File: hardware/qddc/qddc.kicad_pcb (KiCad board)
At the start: 2 copper layers, 71.1 x 46.4 mm, 38 parts, among them IC1 FST3253MTCX, IC2 OPA2350UA, J4 PWR, J7 Conn_01x03_Male, T1 ETC4-1-2TR

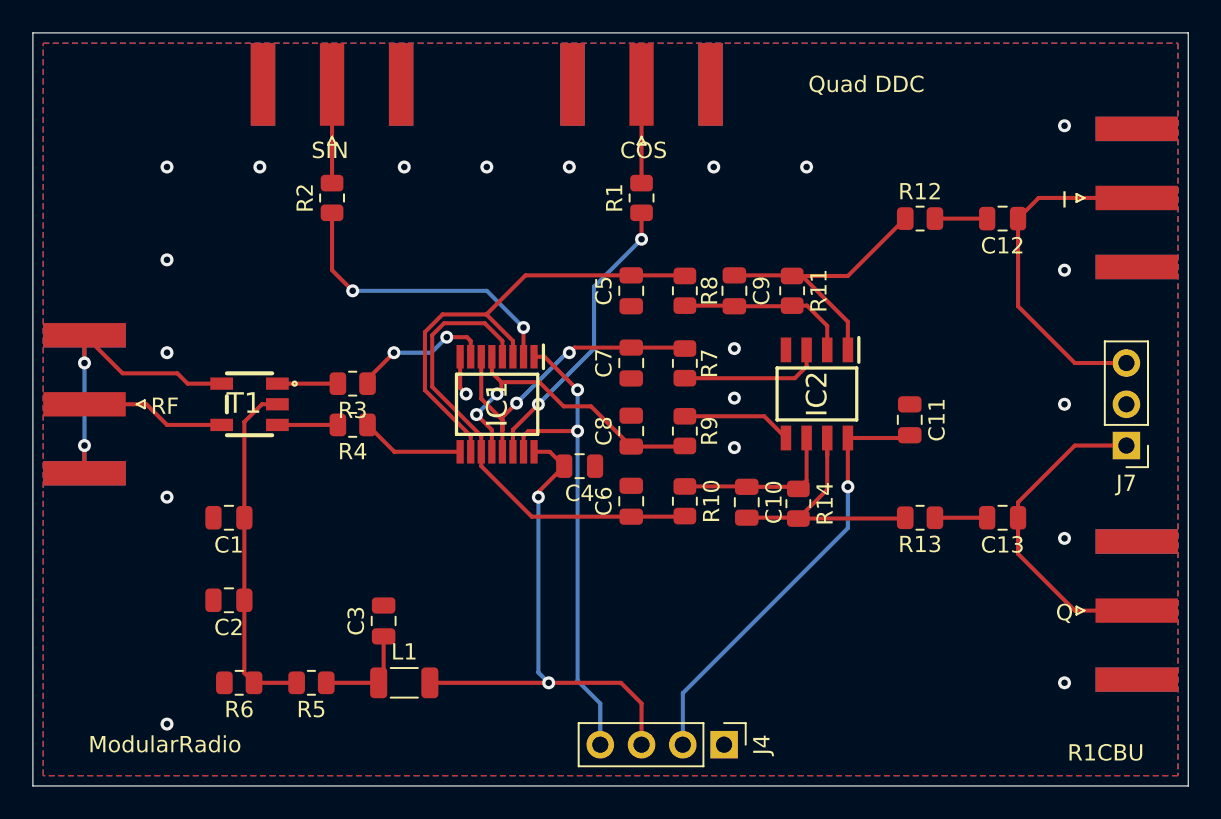
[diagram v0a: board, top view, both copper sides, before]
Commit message: Optimize Quad DDC, Gerber files
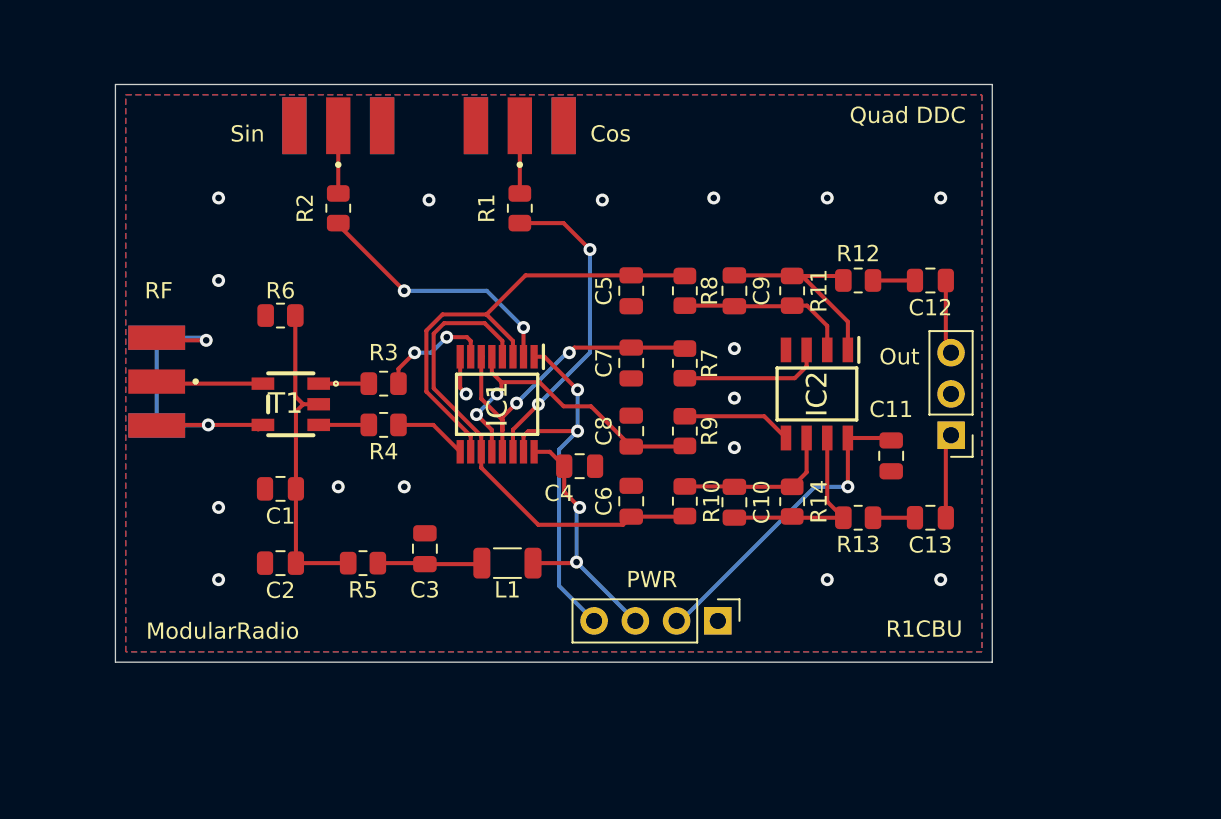
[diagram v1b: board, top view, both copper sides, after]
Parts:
- removed I: Out_I, Connector_Coaxial:SMA_Amphenol_132289_EdgeMount
- removed Q: Out_Q, Connector_Coaxial:SMA_Amphenol_132289_EdgeMount
- removed the RF at (99.7, 106.0)
- added RF: In_RF, kicad:RFSOLUTIONS_CON-SMA-EDGE-S, F.Cu at (104.1, 104.6)
- Cos: renamed from COS; footprint Connector_Coaxial:SMA_Amphenol_132289_EdgeMount -> kicad:RFSOLUTIONS_CON-SMA-EDGE-S
- Sin: renamed from SIN; footprint Connector_Coaxial:SMA_Amphenol_132289_EdgeMount -> kicad:RFSOLUTIONS_CON-SMA-EDGE-S
- moved R6 22.7 mm to (111.8, 100.6)
- moved Out 10.8 mm to (153.0, 108.0)
- moved L1 9.73 mm to (125.7, 115.8)
- moved R5 8.02 mm to (116.8, 115.8)
- moved Cos 7.91 mm to (126.5, 88.9), turned to 270 degrees
- moved PWR 7.63 mm to (138.7, 119.4)
- moved R1 7.52 mm to (126.5, 94.0)
- moved C12 5.85 mm to (151.8, 98.4)
- moved R12 5.39 mm to (147.3, 98.4)
- moved C3 5.12 mm to (120.7, 114.9)
- moved C13 4.45 mm to (151.8, 113.0)
- moved C2 3.91 mm to (111.8, 115.8)
- moved R13 3.81 mm to (147.3, 113.0)
- moved C1 3.64 mm to (111.8, 111.3)
- moved Sin 2.57 mm to (115.3, 88.9), turned to 270 degrees
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- renumbered J7 to Out, J4 to PWR
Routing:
- net Net-(C12-Pad1): track 21.3 -> 4.58 mm
- net VCC: track 32.6 -> 16.4 mm
- net Net-(C13-Pad1): track 20.0 -> 5.21 mm
- net Net-(J3-Pad1): track 21.6 -> 6.95 mm, vias 2 -> 0
- net Net-(J3-PadG1): track 8.97 -> 22.1 mm, vias 0 -> 2
- net VAA: track 27.0 -> 19.9 mm
- net PTT: track 30.4 -> 23.5 mm
- net Net-(C9-Pad1): track 18.3 -> 13.2 mm
- net Net-(C10-Pad2): track 16.6 -> 12.2 mm
- net Net-(IC1-Pad2): track 18.6 -> 15.9 mm
- net Net-(IC1-Pad9): track 6.39 -> 4.48 mm
- net Net-(J2-Pad1): track 6.07 -> 4.23 mm
- net Net-(C1-Pad1): track 21.4 -> 19.8 mm
- net Net-(J1-Pad1): track 6.07 -> 4.46 mm
- net Net-(IC1-Pad7): track 8.77 -> 7.24 mm
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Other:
- board size 71.1 x 46.4 mm -> 54 x 35.6 mm
